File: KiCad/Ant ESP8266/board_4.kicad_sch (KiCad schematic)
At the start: 13 parts

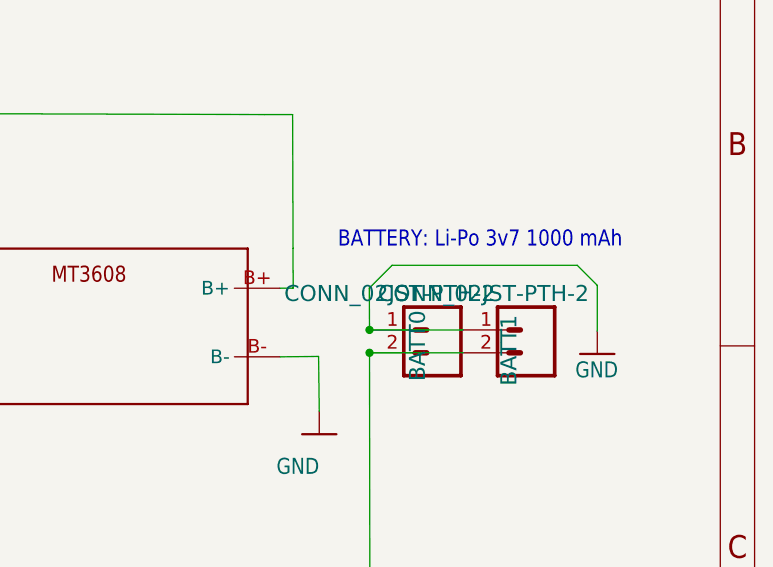
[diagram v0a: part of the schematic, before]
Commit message: Mensaje describiendo tus cambios
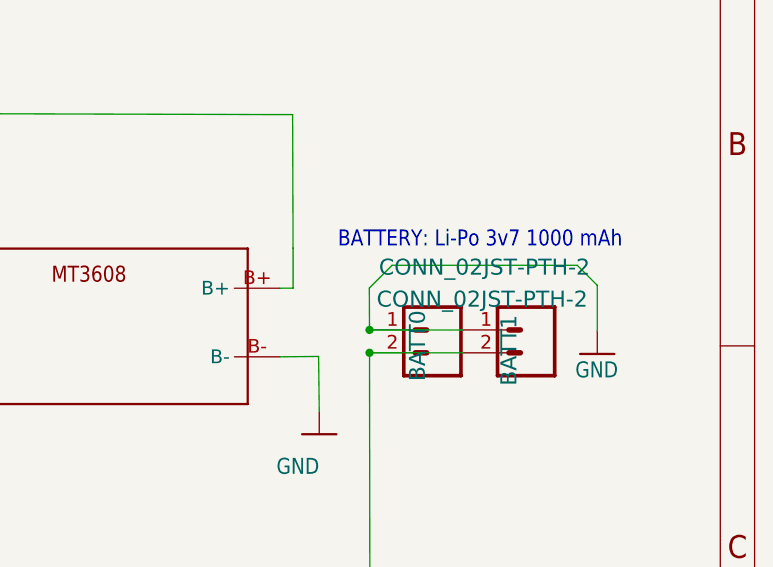
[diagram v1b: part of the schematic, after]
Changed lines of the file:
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@@
 		)
 		(property "Value" "CONN_02JST-PTH-2"
-			(at 249.3146 101.7318 0)
+			(at 259.588 102.362 0)
 			(effects
 				(font
@@
 		)
 		(property "Value" "CONN_02JST-PTH-2"
-			(at 259.7286 101.7318 0)
-			(effects
-				(font
+			(at 259.842 98.806 0)
+			(effects
+				(font
